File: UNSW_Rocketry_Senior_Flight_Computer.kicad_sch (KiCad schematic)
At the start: 19 parts, among them U1 STM32L452RETx, U2 MS5611-01BA, U3 MS5611-01BA, U4 LIS3DH, Y1 8MHz

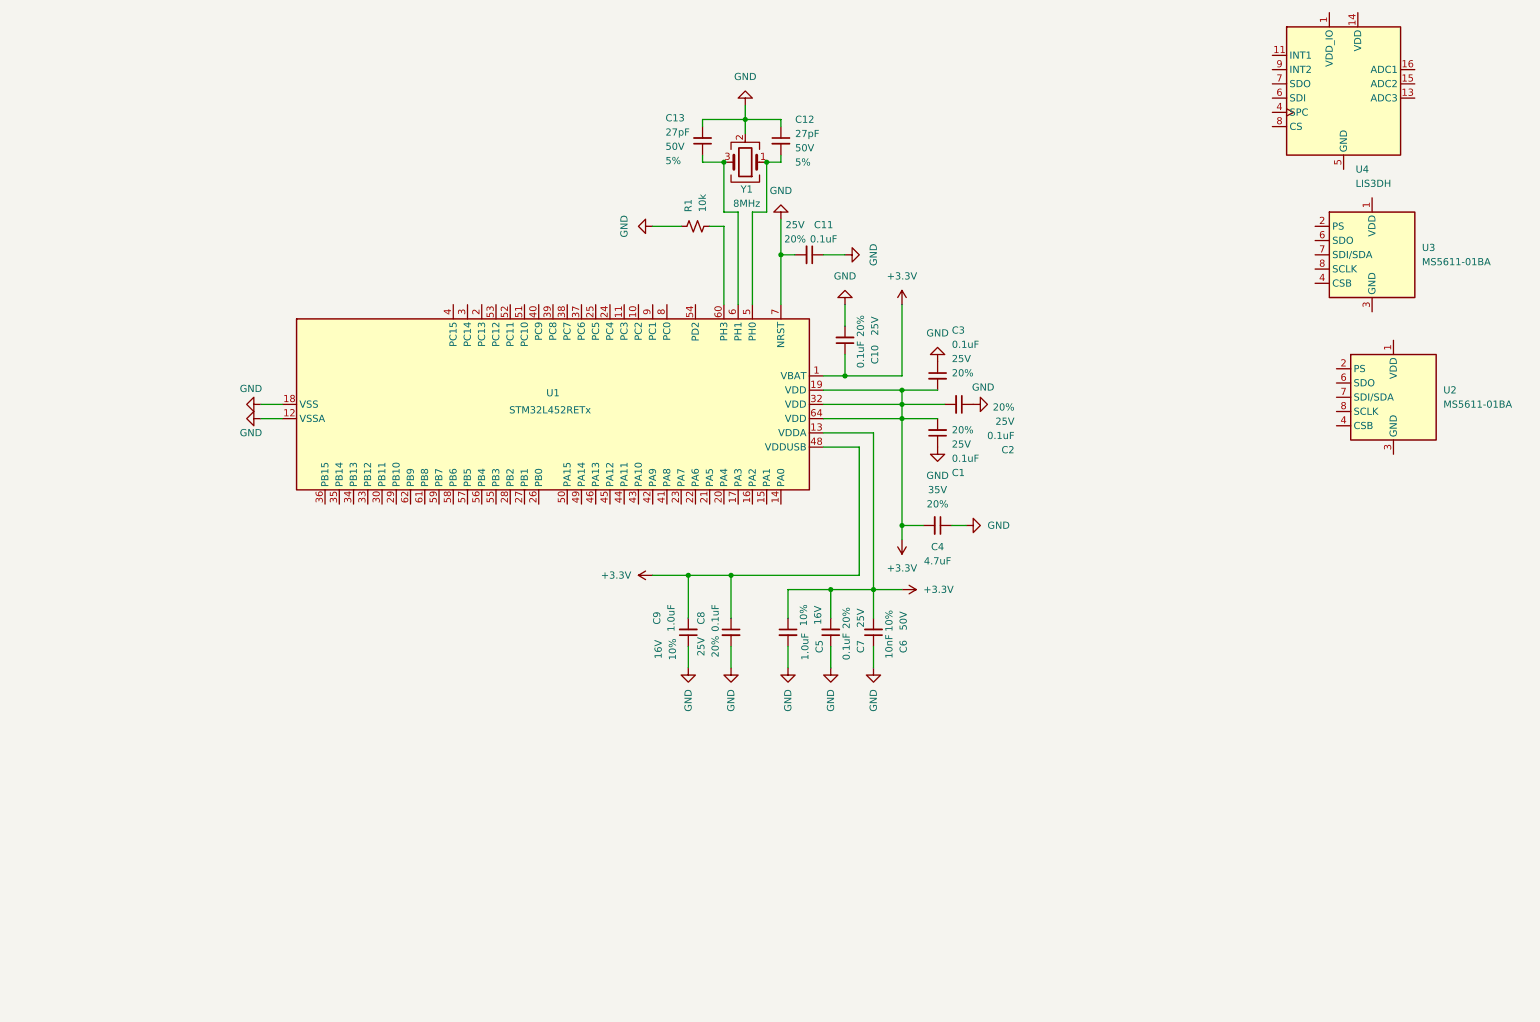
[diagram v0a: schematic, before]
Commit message: feat: Power & comms
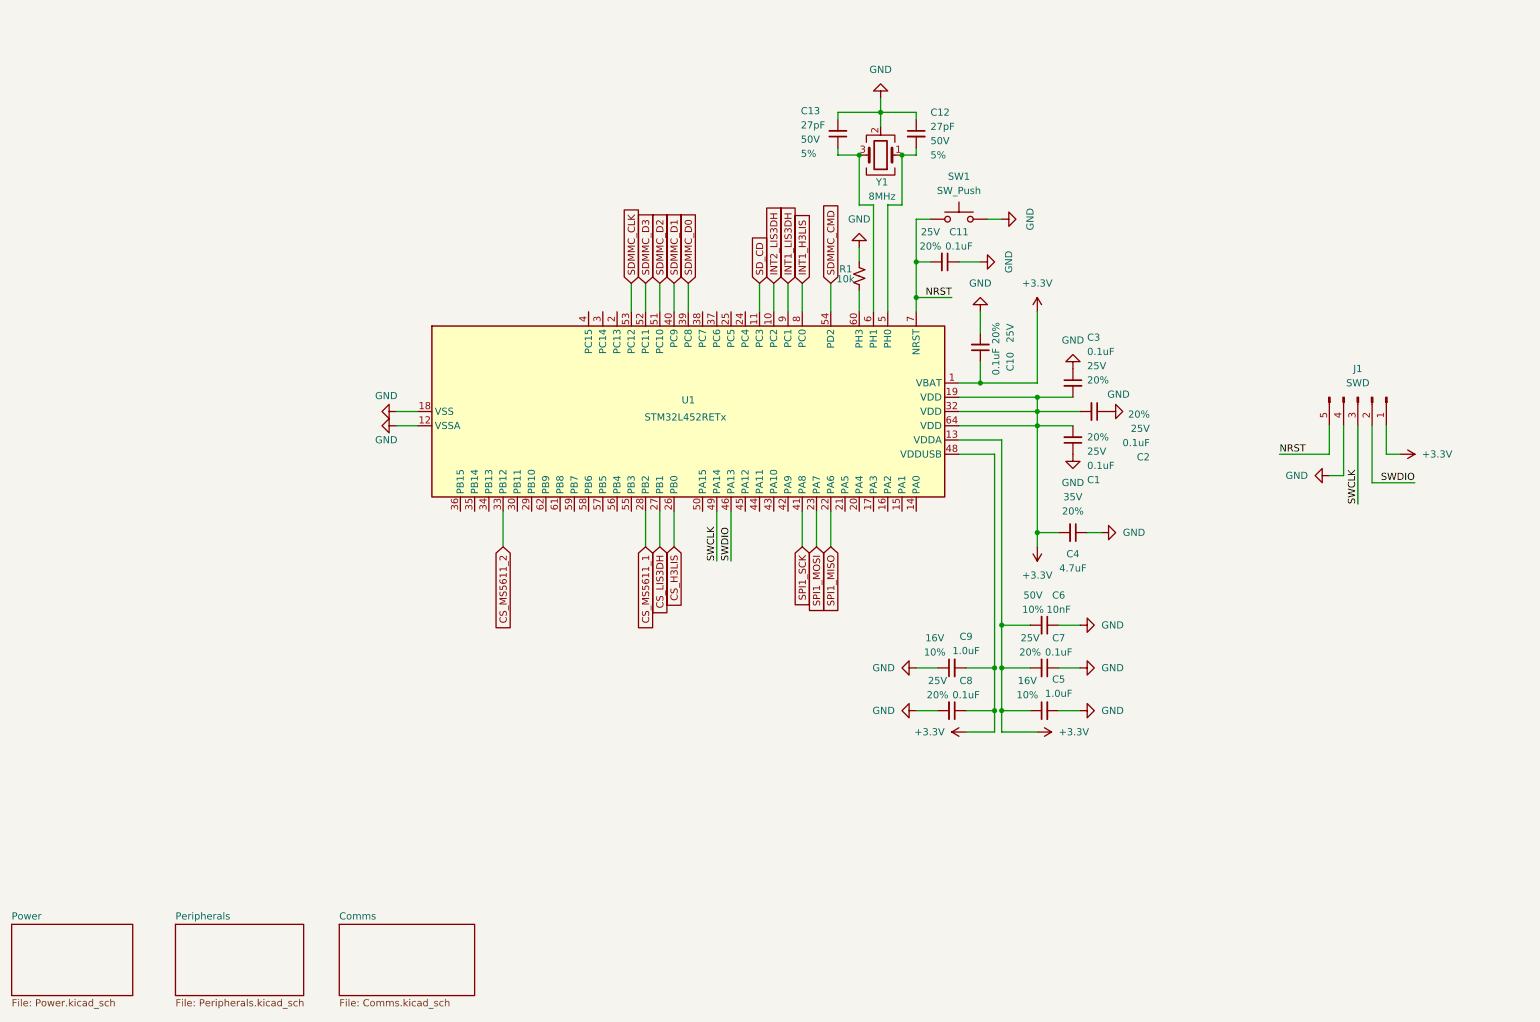
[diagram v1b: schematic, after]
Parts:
- removed U2, U3: MS5611-01BA, Package_LGA:LGA-8_3x5mm_P1.25mm, symbol Sensor_Pressure:MS5611-01BA
- removed U4: LIS3DH, Package_LGA:LGA-16_3x3mm_P0.5mm_LayoutBorder3x5y, symbol Sensor_Motion:LIS3DH
- added J1: SWD, Connector_PinHeader_2.54mm:PinHeader_1x05_P2.54mm_Vertical, symbol Connector:Conn_01x05_Pin
- added SW1: SW_Push, Button_Switch_SMD:SW_SPST_PTS645Sx43SMTR92, symbol Switch:SW_Push
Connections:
- net +3.3V: now also J1.1 (Pin_1)
- net GND: now also J1.4 (Pin_4), SW1.2; no longer C11.2, U1.7 (NRST)
- net INT2_LIS3DH: now reaches U1.10 (PC2)
- net SD_CD: now reaches U1.11 (PC3)
- net SPI1_MISO: now reaches U1.22 (PA6)
- net SPI1_MOSI: now reaches U1.23 (PA7)
- net CS_H3LIS: now reaches U1.26 (PB0)
- net CS_LIS3DH: now reaches U1.27 (PB1)
- net CS_MS5611_1: now reaches U1.28 (PB2)
- net CS_MS5611_2: now reaches U1.33 (PB12)
- net SDMMC_D0: now reaches U1.39 (PC8)
- net SDMMC_D1: now reaches U1.40 (PC9)
- net SPI1_SCK: now reaches U1.41 (PA8)
- net SWDIO: now reaches U1.46 (PA13)
- net SWDIO: now also J1.2 (Pin_2)
- net SWCLK: now reaches U1.49 (PA14)
- net SWCLK: now also J1.3 (Pin_3)
- net SDMMC_D2: now reaches U1.51 (PC10)
- net SDMMC_D3: now reaches U1.52 (PC11)
- net SDMMC_CLK: now reaches U1.53 (PC12)
- net SDMMC_CMD: now reaches U1.54 (PD2)
- net INT1_H3LIS: now reaches U1.8 (PC0)
- net INT1_LIS3DH: now reaches U1.9 (PC1)
- new net NRST: C11.2, J1.5 (Pin_5), SW1.1, U1.7 (NRST)
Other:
- added sheet Comms (Comms.kicad_sch)
- added sheet Peripherals (Peripherals.kicad_sch)
- added sheet Power (Power.kicad_sch)
- moved on the sheet: C1, C10, C11, C12, C13, C2, C3, C4, C5, C6, C7, C8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

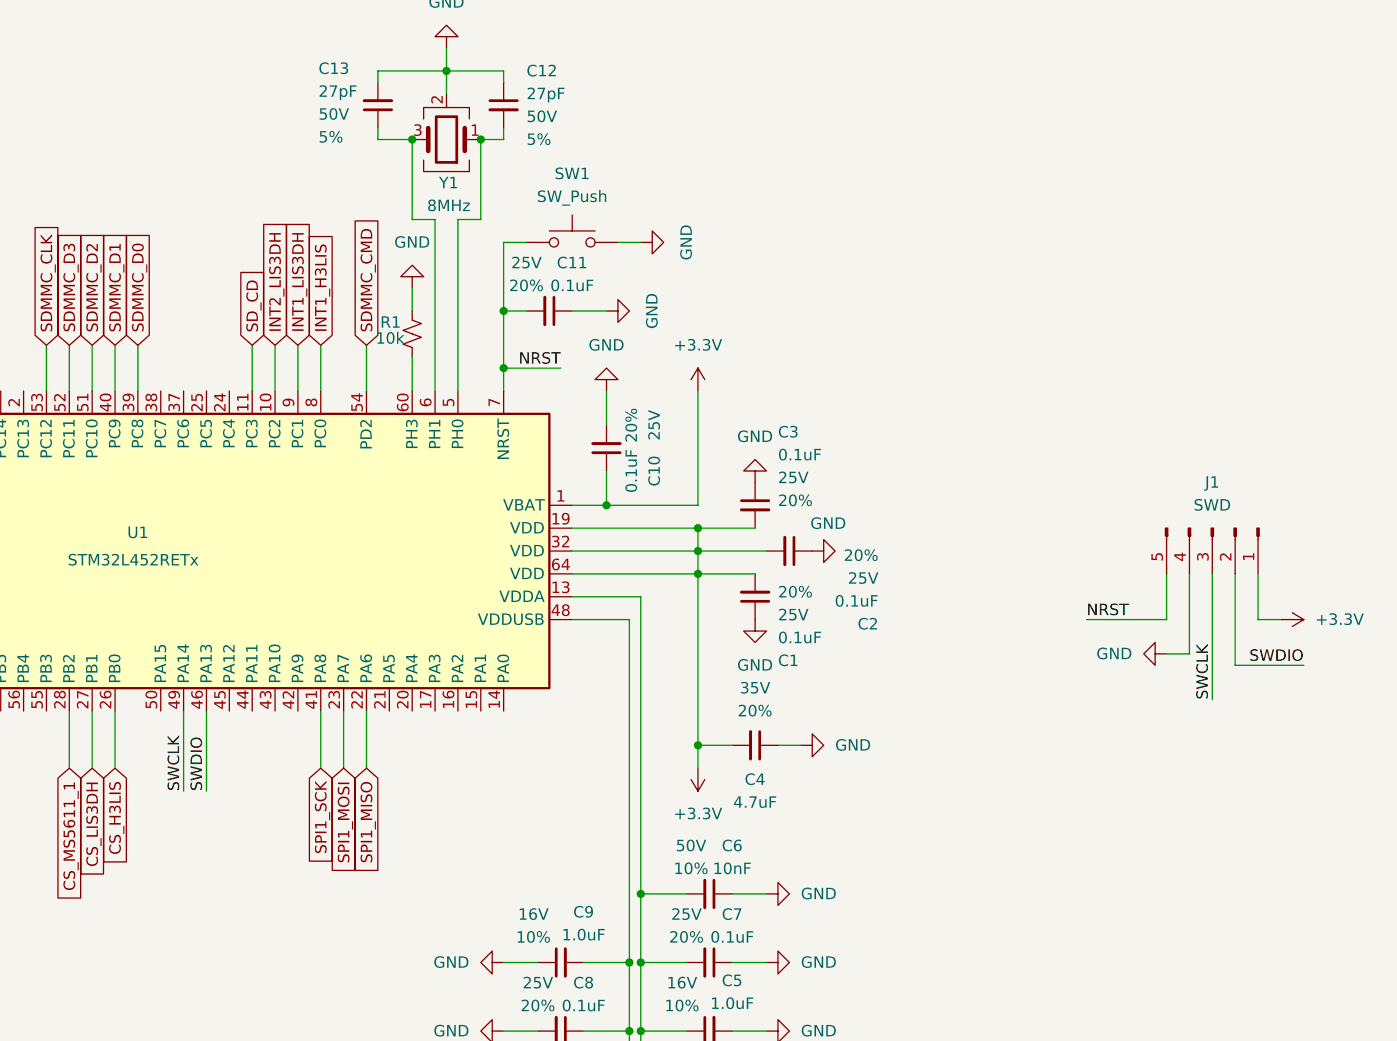
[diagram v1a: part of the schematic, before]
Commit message: feat: Comms complete
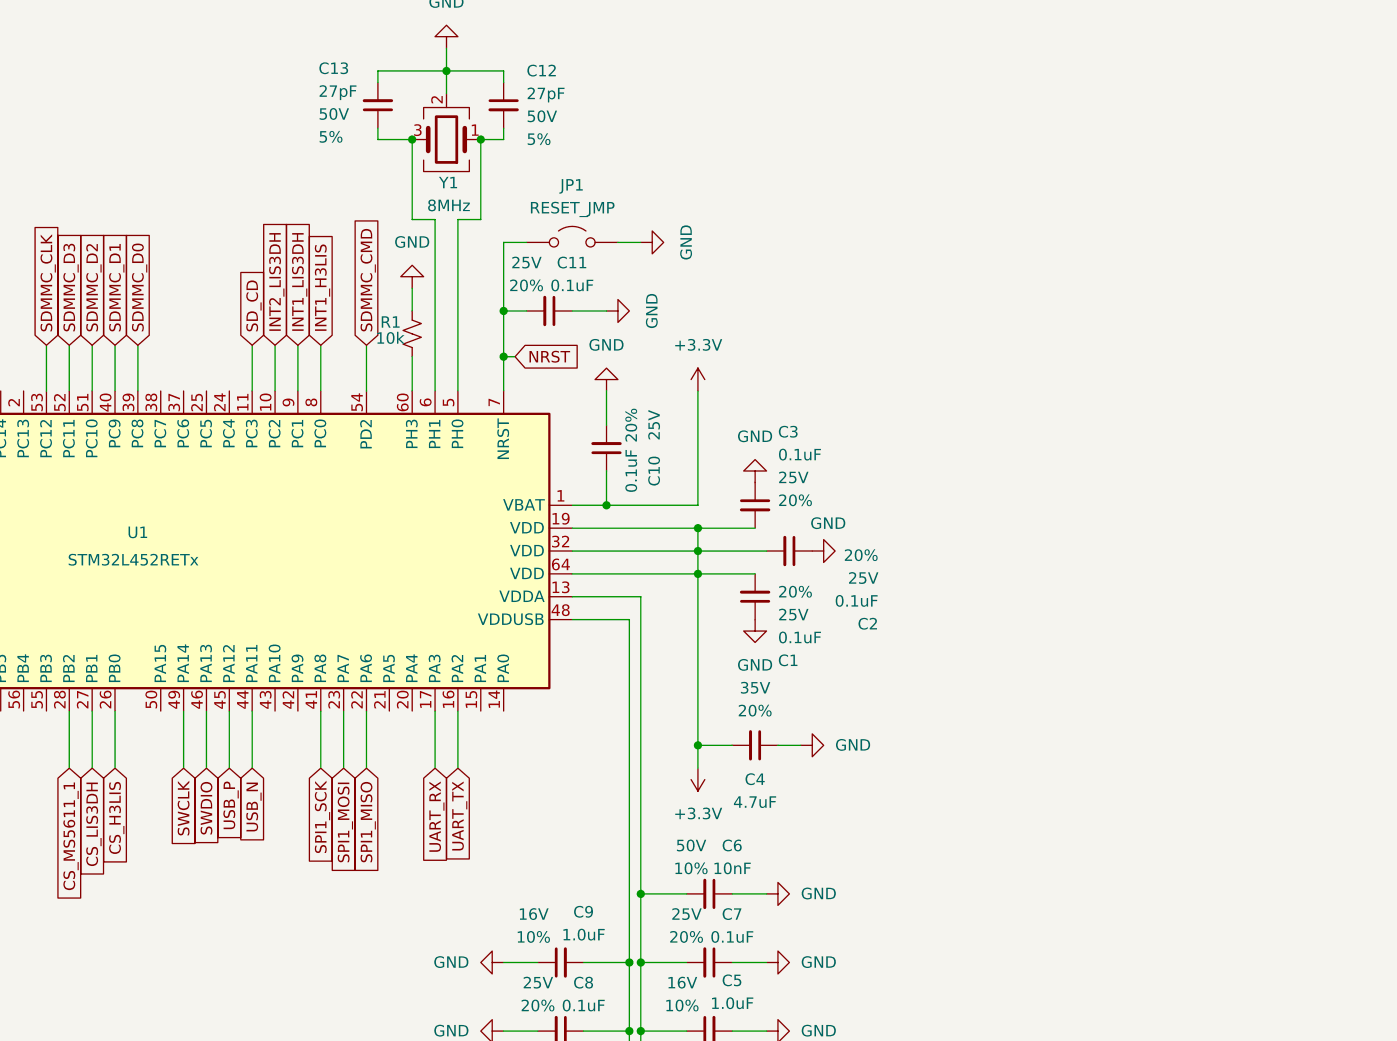
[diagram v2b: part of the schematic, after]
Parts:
- removed J1: SWD, Connector_PinHeader_2.54mm:PinHeader_1x05_P2.54mm_Vertical, symbol Connector:Conn_01x05_Pin
- removed SW1: SW_Push, Button_Switch_SMD:SW_SPST_PTS645Sx43SMTR92, symbol Switch:SW_Push
- added JP1: RESET_JMP, TestPoint:TestPoint_2Pads_Pitch2.54mm_Drill0.8mm, symbol Jumper:Jumper_2_Open
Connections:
- net GND: now also JP1.2 (B)
- net NRST: now also JP1.1 (A)
- net UART_TX: now reaches U1.16 (PA2)
- net UART_RX: now reaches U1.17 (PA3)
- net USB_N: now reaches U1.44 (PA11)
- net USB_P: now reaches U1.45 (PA12)

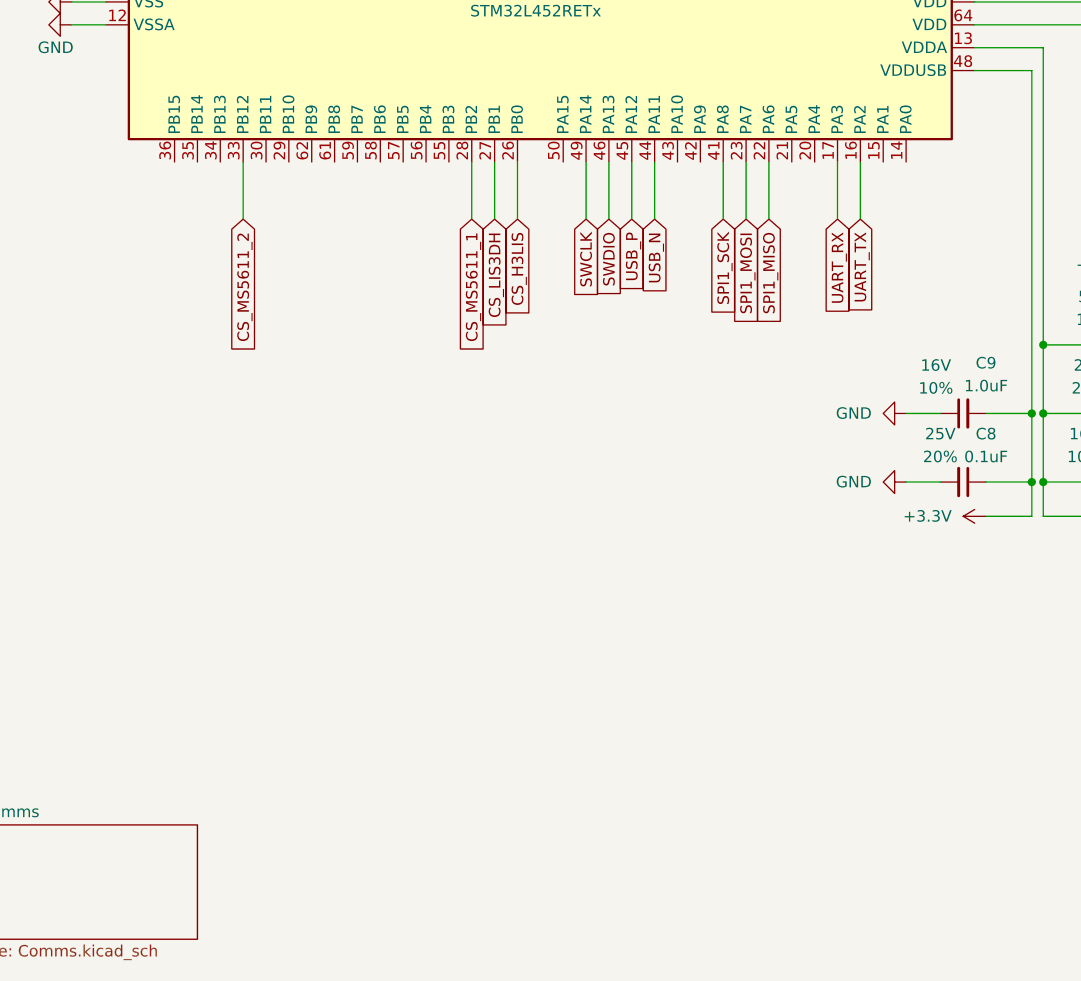
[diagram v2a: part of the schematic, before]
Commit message: feat: Pyro done
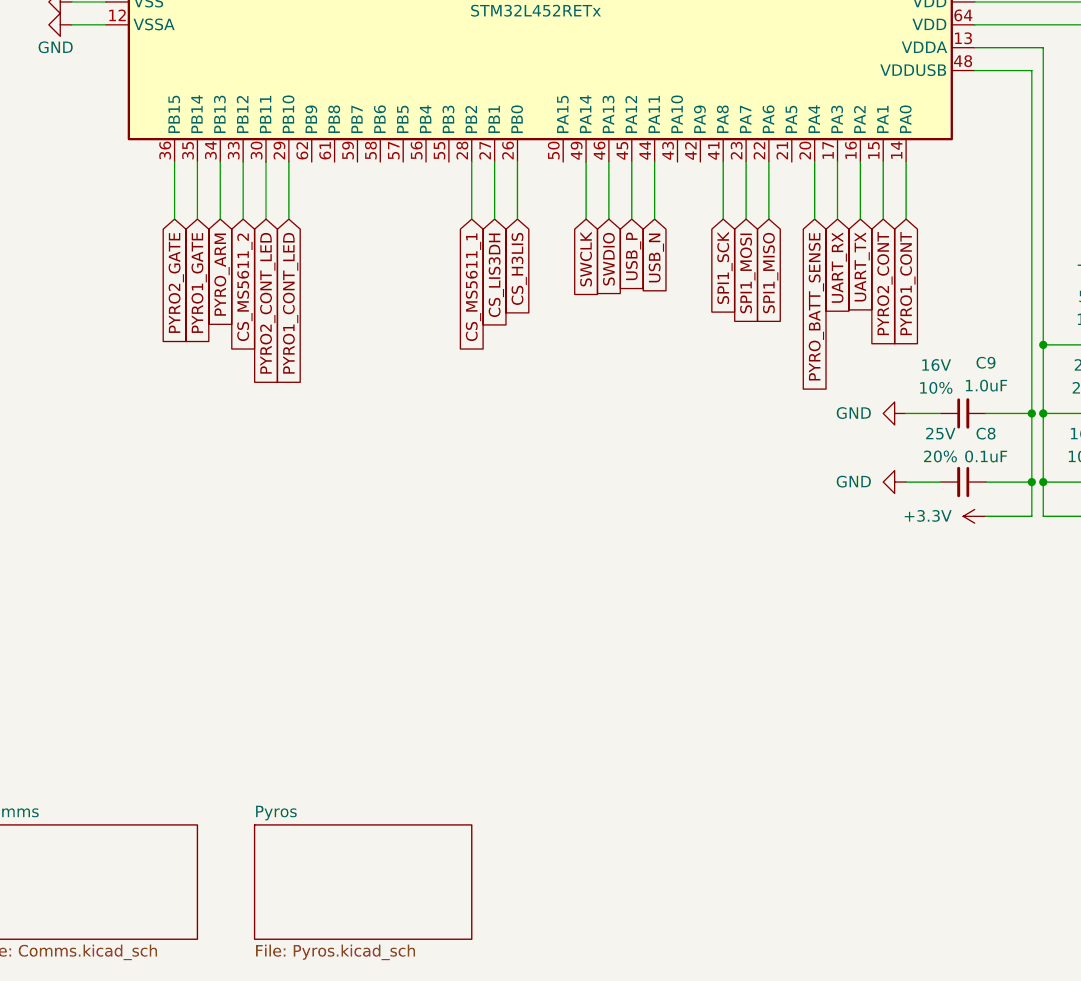
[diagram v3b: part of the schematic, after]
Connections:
- net PYRO1_CONT: now reaches U1.14 (PA0)
- net PYRO2_CONT: now reaches U1.15 (PA1)
- net PYRO_BATT_SENSE: now reaches U1.20 (PA4)
- net PYRO1_CONT_LED: now reaches U1.29 (PB10)
- net PYRO2_CONT_LED: now reaches U1.30 (PB11)
- net PYRO_ARM: now reaches U1.34 (PB13)
- net PYRO1_GATE: now reaches U1.35 (PB14)
- net PYRO2_GATE: now reaches U1.36 (PB15)
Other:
- added sheet Pyros (Pyros.kicad_sch)
